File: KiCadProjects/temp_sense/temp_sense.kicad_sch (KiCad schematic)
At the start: 14 parts, among them J1 Screw_Terminal_01x02, J2 Screw_Terminal_01x02, J3 Conn_01x02_Pin, J4 Conn_01x03_Pin, U1 ADS1115IDGS, U2 TLV70033_SOT23-5

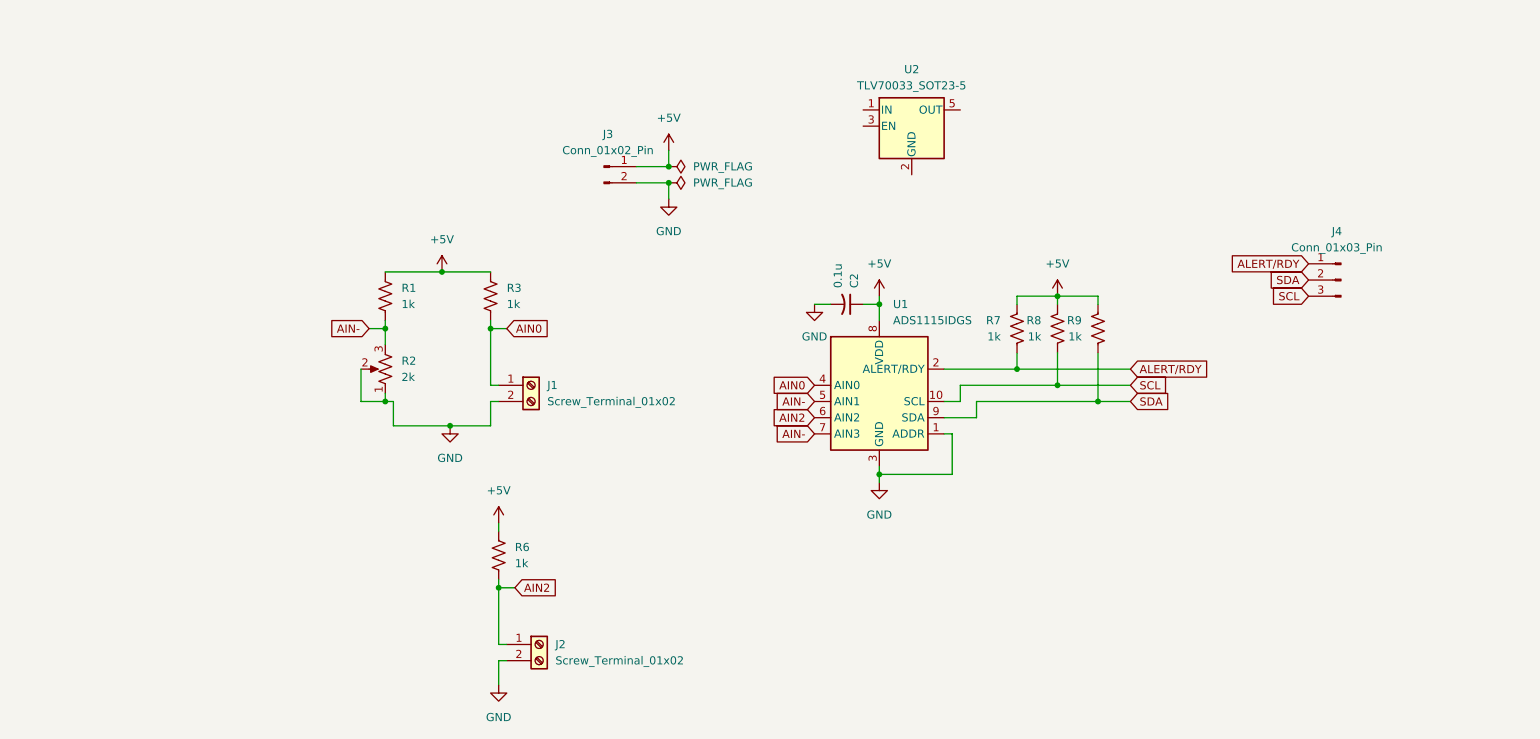
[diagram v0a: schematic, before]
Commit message: finish evm board
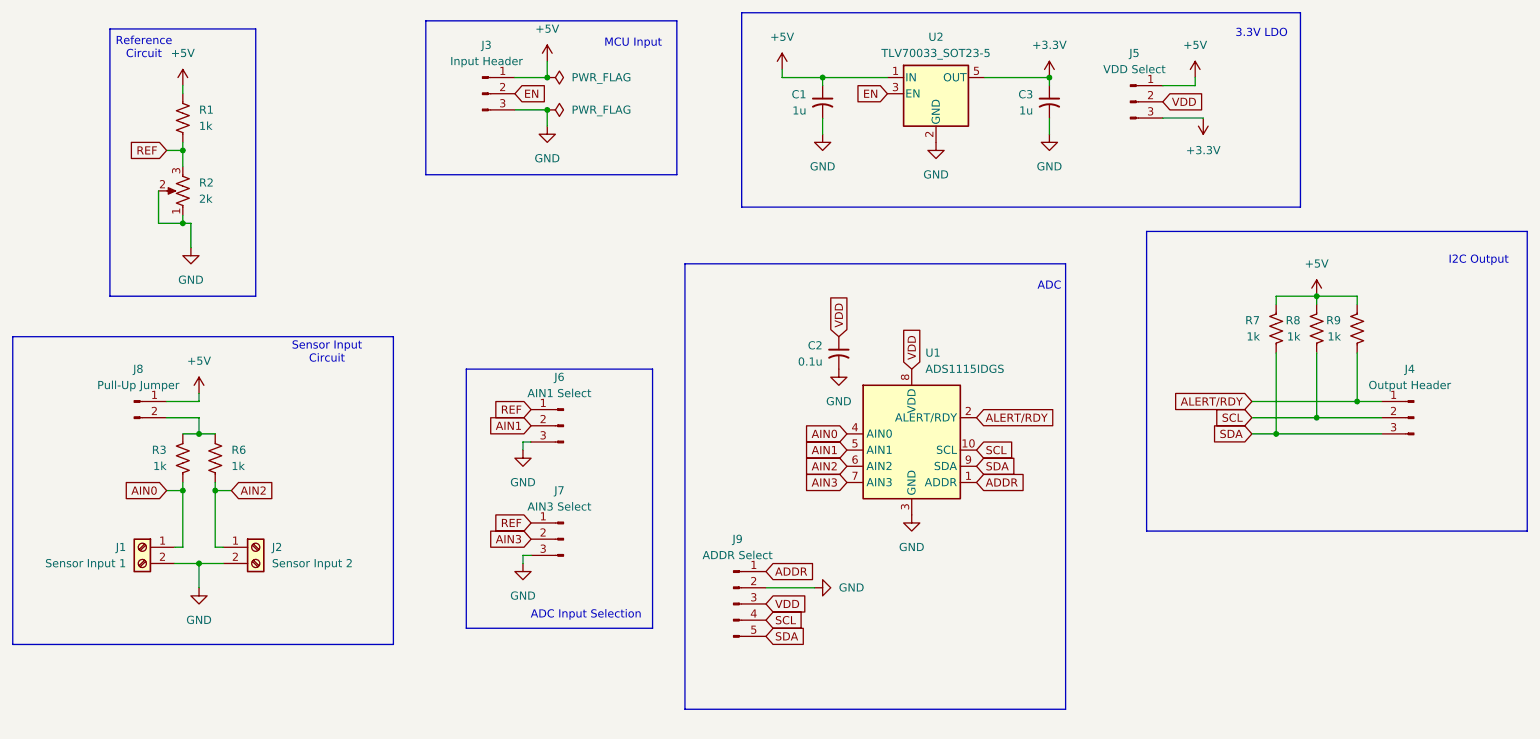
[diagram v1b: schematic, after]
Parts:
- removed J3: Conn_01x02_Pin, Connector_PinHeader_2.54mm:PinHeader_1x02_P2.54mm_Vertical, symbol Connector:Conn_01x02_Pin
- added C1, C3: 1u, Capacitor_SMD:C_0201_0603Metric_Pad0.64x0.40mm_HandSolder, symbol Device:C_Small_US
- added J3: Input Header, Connector_PinHeader_2.54mm:PinHeader_1x03_P2.54mm_Vertical, symbol Connector:Conn_01x03_Pin
- added J5: VDD Select, Connector_PinHeader_2.54mm:PinHeader_1x03_P2.54mm_Vertical, symbol Connector:Conn_01x03_Pin
- added J6: AIN1 Select, Connector_PinHeader_2.54mm:PinHeader_1x03_P2.54mm_Vertical, symbol Connector:Conn_01x03_Pin
- added J7: AIN3 Select, Connector_PinHeader_2.54mm:PinHeader_1x03_P2.54mm_Vertical, symbol Connector:Conn_01x03_Pin
- added J8: Pull-Up Jumper, Connector_PinHeader_2.54mm:PinHeader_1x02_P2.54mm_Vertical, symbol Connector:Conn_01x02_Pin
- added J9: ADDR Select, Connector_PinHeader_2.54mm:PinHeader_1x05_P2.54mm_Vertical, symbol Connector:Conn_01x05_Pin
- J1: value Screw_Terminal_01x02 -> Sensor Input 1
- J2: value Screw_Terminal_01x02 -> Sensor Input 2
- J4: value Conn_01x03_Pin -> Output Header
- U2: LCSC (none) -> C11337; Link (none) -> https://www.lcsc.com/product-detail/C11337.html?s_z=h_tlv70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
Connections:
- net +5V: now also U2.1 (IN), C1.1, J3.1 (Pin_1), J5.1 (Pin_1), J8.1 (Pin_1); no longer C2.1, R3.1, R6.1, U1.8 (VDD)
- net ALERT/RDY: now also R9.2; no longer R7.2
- net GND: now also U2.2 (GND), C1.2, C3.2, J3.3 (Pin_3), J6.3 (Pin_3), J7.3 (Pin_3), J9.2 (Pin_2); no longer U1.1 (ADDR)
- net SCL: now also J4.2 (Pin_2), J9.4 (Pin_4); no longer J4.3 (Pin_3)
- net SDA: now also J4.3 (Pin_3), R7.2, J9.5 (Pin_5); no longer J4.2 (Pin_2), R9.2
- net EN: now reaches U2.3 (EN)
- net EN: now also J3.2 (Pin_2)
- net +3.3V: now reaches U2.5 (OUT)
- net +3.3V: now also C3.1, J5.3 (Pin_3)
- net AIN- renamed REF
- net REF: now also J6.1 (Pin_1), J7.1 (Pin_1); no longer U1.5 (AIN1), U1.7 (AIN3)
- new net: J8.2 (Pin_2), R3.1, R6.1
- new net ADDR: J9.1 (Pin_1), U1.1 (ADDR)
- new net AIN1: J6.2 (Pin_2), U1.5 (AIN1)
- new net AIN3: J7.2 (Pin_2), U1.7 (AIN3)
- new net VDD: C2.1, J5.2 (Pin_2), J9.3 (Pin_3), U1.8 (VDD)
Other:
- note added: "3.3V LDO"
- note added: "ADC"
- note added: "ADC Input Selection"
- note added: "I2C Output"
- note added: "MCU Input"
- note added: "Reference Circuit"
- note added: "Sensor Input Circuit"
- moved on the sheet: C2, J1, J2, J4, R1, R2, R3, R6, R7, R8, R9, U1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

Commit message: temp sense rev 2
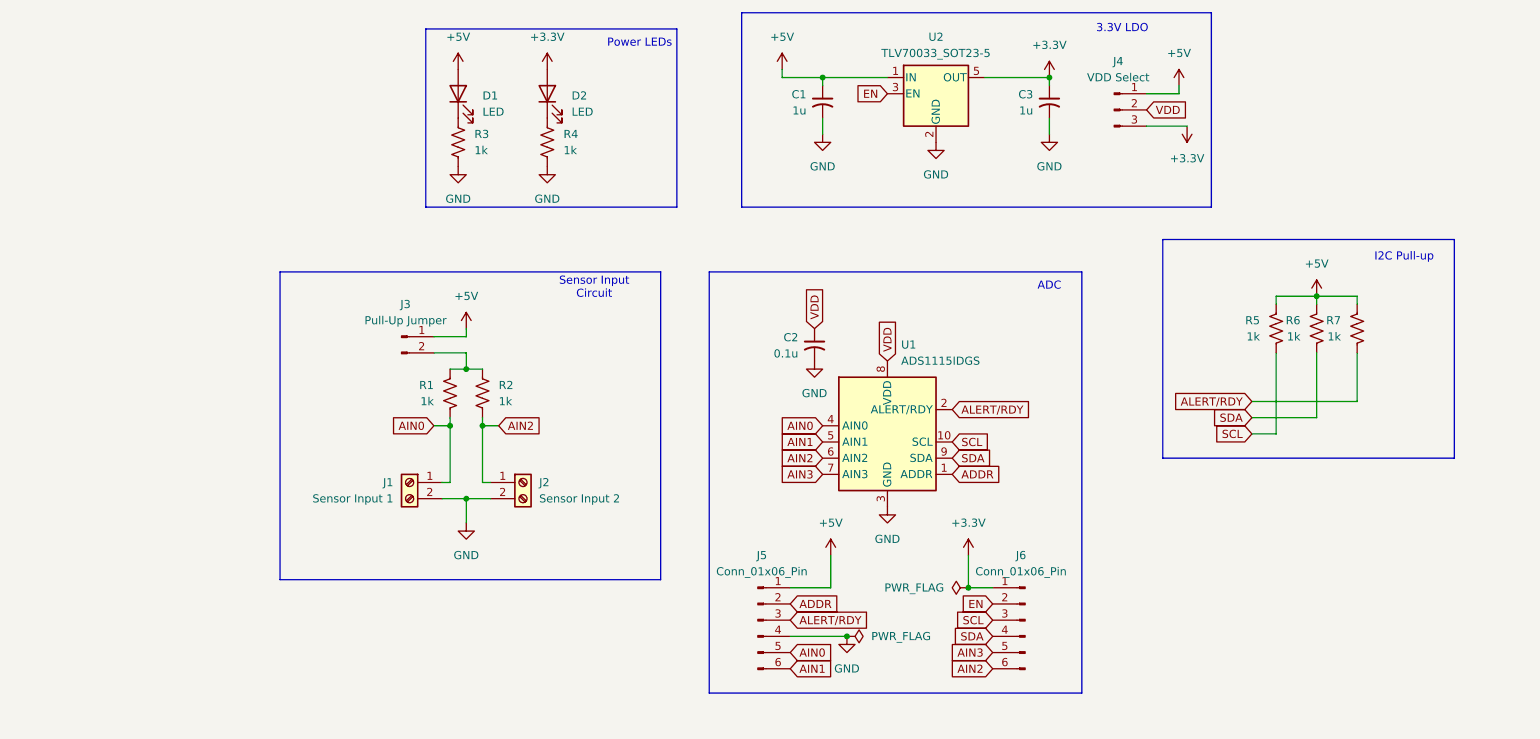
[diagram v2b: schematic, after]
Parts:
- removed J3: Input Header, Connector_PinHeader_2.54mm:PinHeader_1x03_P2.54mm_Vertical, symbol Connector:Conn_01x03_Pin
- removed J4: Output Header, Connector_PinHeader_2.54mm:PinHeader_1x03_P2.54mm_Vertical, symbol Connector:Conn_01x03_Pin
- removed J6: AIN1 Select, Connector_PinHeader_2.54mm:PinHeader_1x03_P2.54mm_Vertical, symbol Connector:Conn_01x03_Pin
- removed J7: AIN3 Select, Connector_PinHeader_2.54mm:PinHeader_1x03_P2.54mm_Vertical, symbol Connector:Conn_01x03_Pin
- removed J9: ADDR Select, Connector_PinHeader_2.54mm:PinHeader_1x05_P2.54mm_Vertical, symbol Connector:Conn_01x05_Pin
- removed R1: 1k, Resistor_SMD:R_0201_0603Metric_Pad0.64x0.40mm_HandSolder, symbol Device:R_US
- removed R2: 2k, 0_project:POT_PV36W_MUR, symbol Device:R_Potentiometer_US
- added D1, D2: LED, LED_SMD:LED_0603_1608Metric, symbol Device:LED
- added J5, J6: Conn_01x06_Pin, Connector_PinHeader_2.54mm:PinHeader_1x06_P2.54mm_Vertical, symbol Connector:Conn_01x06_Pin
- added R3, R4: 1k, Resistor_SMD:R_0603_1608Metric_Pad0.98x0.95mm_HandSolder, symbol Device:R_US
- C1, C2, C3: footprint Capacitor_SMD:C_0201_0603Metric_Pad0.64x0.40mm_HandSolder -> Capacitor_SMD:C_0603_1608Metric_Pad1.08x0.95mm_HandSolder
- R1: renamed from R3; footprint Resistor_SMD:R_0201_0603Metric_Pad0.64x0.40mm_HandSolder -> Resistor_SMD:R_0603_1608Metric_Pad0.98x0.95mm_HandSolder
- R2: renamed from R6; footprint Resistor_SMD:R_0201_0603Metric_Pad0.64x0.40mm_HandSolder -> Resistor_SMD:R_0603_1608Metric_Pad0.98x0.95mm_HandSolder
- R5: renamed from R7; footprint Resistor_SMD:R_0201_0603Metric_Pad0.64x0.40mm_HandSolder -> Resistor_SMD:R_0603_1608Metric_Pad0.98x0.95mm_HandSolder
- R6: renamed from R8; footprint Resistor_SMD:R_0201_0603Metric_Pad0.64x0.40mm_HandSolder -> Resistor_SMD:R_0603_1608Metric_Pad0.98x0.95mm_HandSolder
- R7: renamed from R9; footprint Resistor_SMD:R_0201_0603Metric_Pad0.64x0.40mm_HandSolder -> Resistor_SMD:R_0603_1608Metric_Pad0.98x0.95mm_HandSolder
- renumbered J8 to J3, J5 to J4
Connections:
- net +3.3V: now also D2.2 (A), J6.1 (Pin_1)
- net +5V: now also D1.2 (A), J5.1 (Pin_1)
- net ADDR: now also J5.2 (Pin_2)
- net AIN0: now also J5.5 (Pin_5)
- net AIN1: now also J5.6 (Pin_6)
- net AIN2: now also J6.6 (Pin_6)
- net AIN3: now also J6.5 (Pin_5)
- net ALERT/RDY: now also J5.3 (Pin_3)
- net EN: now also J6.2 (Pin_2)
- net GND: now also J5.4 (Pin_4), R3.2, R4.2
- net SCL: now also R5.2, J6.3 (Pin_3); no longer R6.2
- net SDA: now also R6.2, J6.4 (Pin_4); no longer R5.2
- new net: D1.1 (K), R3.1
- new net: D2.1 (K), R4.1
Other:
- note added: "I2C Pull-up"
- note added: "Power LEDs"
- note removed: "ADC Input Selection"
- note removed: "I2C Output"
- note removed: "MCU Input"
- note removed: "Reference Circuit"
- moved on the sheet: C2, J1, J2, J3, J4, R1, R2, U1
